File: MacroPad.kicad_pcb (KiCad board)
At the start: 2 copper layers, 111.1 x 120.1 mm, 56 parts, among them J1 AVR-ISP-6, SW1 Rotary_Encoder_Switch, SW10 *, SW11 9, SW12 6, SW13 3, SW14 ., SW15 -, SW16 +, SW17 Enter, SW18 SW_Push, SW2 7, SW3 4, SW4 1, SW5 0, SW6 /, SW7 8, SW8 5, SW9 2, U1 ATmega32U4-AU, U2 PRTR5V0U2X, Y1 16Mhz

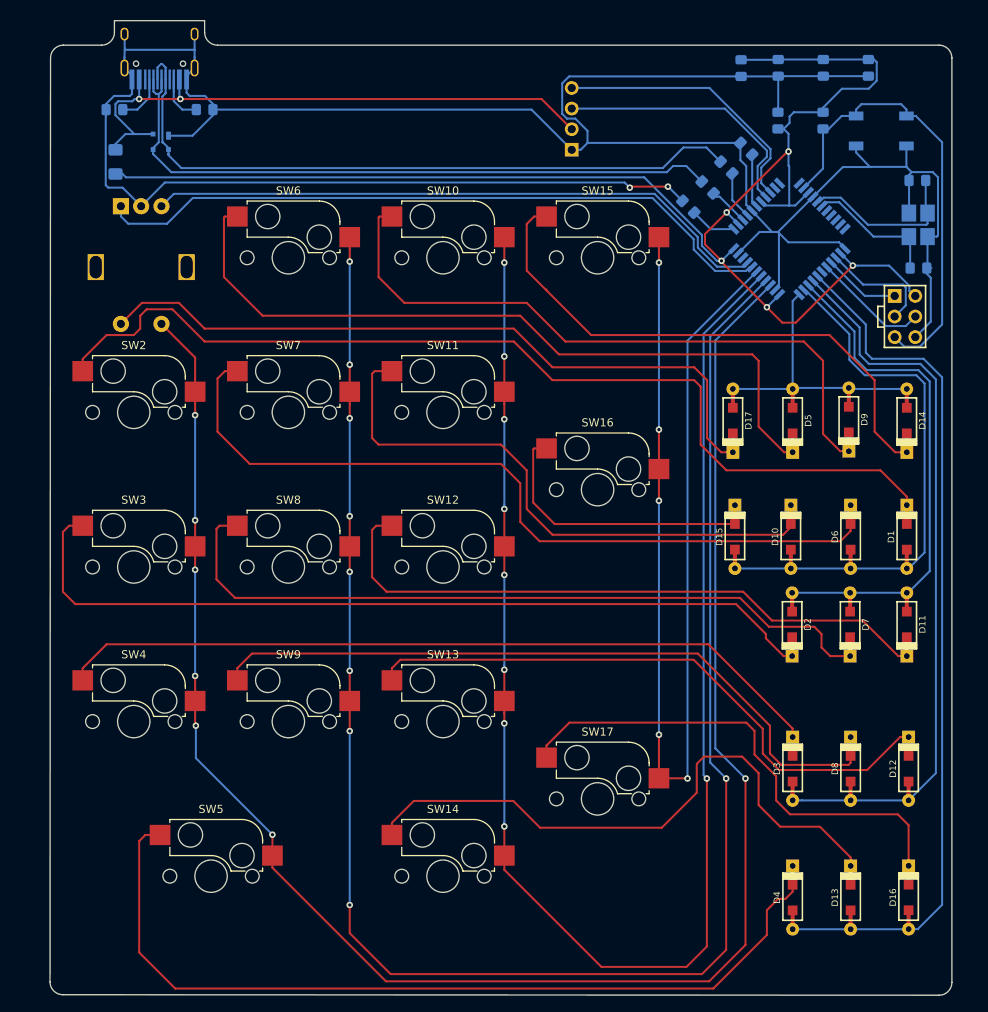
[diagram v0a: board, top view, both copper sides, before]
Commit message: cambiando rutas
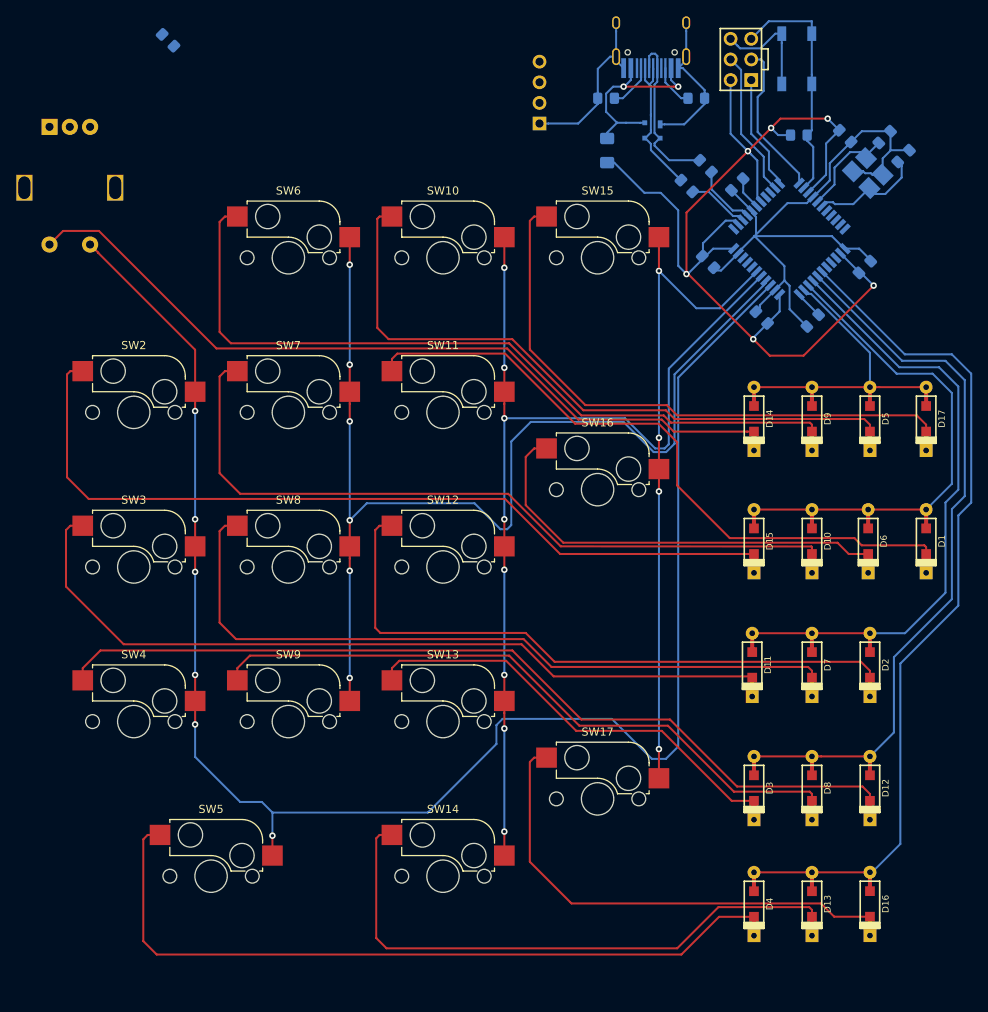
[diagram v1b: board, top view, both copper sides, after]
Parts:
- moved C3 70.7 mm to (54.2, 65.3), turned to 135 degrees
- moved R1 60.6 mm to (119.3, 72.4)
- moved F1 60.6 mm to (108.3, 78.9)
- moved USB1 60.6 mm to (113.8, 60.5)
- moved R2 60.6 mm to (108.2, 72.4)
- moved U2 60.6 mm to (113.9, 76.4)
- moved J1 37.6 mm to (124.8, 67.6), turned to 90 degrees
- moved C2 30.8 mm to (127.4, 99.4), turned to 135 degrees
- moved C5 27.8 mm to (120.8, 92.6), turned to 315 degrees
- moved D17 23.8 mm to (147.6, 111.9)
- moved C4 21.0 mm to (140.1, 93.2), turned to 45 degrees
- moved R6 20.8 mm to (133.7, 99.8), turned to 45 degrees
- moved D11 19.7 mm to (126.2, 142.2)
- moved D14 18.8 mm to (126.4, 111.9)
- moved C6 13.9 mm to (144.9, 79.5), turned to 45 degrees
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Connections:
- net sw14 renamed Net-(D13-Pad1)
- net sw17 renamed Net-(D16-Pad1)
- net sw5 renamed Net-(D4-Pad1)
- net sw8 renamed Net-(D7-Pad1)
- net sw9 renamed Net-(D8-Pad1)
- D1 pad 1: sw2 -> Net-(D1-Pad1)
- D1 pad 2: row1 -> ROW1
- D10 pad 1: sw11 -> Net-(D10-Pad1)
- D10 pad 2: row1 -> ROW1
- D11 pad 1: sw12 -> Net-(D11-Pad1)
- D11 pad 2: row2 -> ROW2
- D12 pad 1: sw13 -> Net-(D12-Pad1)
- D12 pad 2: row3 -> ROW3
- D13 pad 2: row4 -> ROW4
- D14 pad 1: sw15 -> Net-(D14-Pad1)
- D14 pad 2: row0 -> ROW0
- D15 pad 1: sw16 -> Net-(D15-Pad1)
- D15 pad 2: row1 -> ROW1
- D16 pad 2: row4 -> ROW4
- D17 pad 1: S2 -> Net-(D17-Pad1)
- D17 pad 2: row0 -> ROW0
- D2 pad 1: sw3 -> Net-(D2-Pad1)
- D2 pad 2: row2 -> ROW2
- D3 pad 1: sw4 -> Net-(D3-Pad1)
- D3 pad 2: row3 -> ROW3
- D4 pad 2: row4 -> ROW4
- D5 pad 1: sw6 -> Net-(D5-Pad1)
- D5 pad 2: row0 -> ROW0
- D6 pad 1: sw7 -> Net-(D6-Pad1)
- D6 pad 2: row1 -> ROW1
- D7 pad 2: row2 -> ROW2
- D8 pad 2: row3 -> ROW3
- D9 pad 1: sw10 -> Net-(D9-Pad1)
- D9 pad 2: row0 -> ROW0
- SW1 pad S1: col0 -> col3
- SW1 pad S2: S2 -> Net-(D14-Pad1)
- SW10 pad 1: sw10 -> Net-(D5-Pad1)
- SW10 pad 2: col2 -> col1
- SW11 pad 1: sw11 -> Net-(D1-Pad1)
- SW11 pad 2: col2 -> col1
- SW12 pad 1: sw12 -> Net-(D2-Pad1)
- SW12 pad 2: col2 -> col1
- SW13 pad 1: sw13 -> Net-(D3-Pad1)
- SW13 pad 2: col2 -> col1
- SW14 pad 2: col2 -> col1
- SW15 pad 1: sw15 -> Net-(D17-Pad1)
- SW15 pad 2: col3 -> col0
- SW16 pad 1: sw16 -> Net-(D6-Pad1)
- SW16 pad 2: col3 -> col0
- SW17 pad 2: col3 -> col0
- SW2 pad 1: sw2 -> Net-(D15-Pad1)
- SW2 pad 2: col0 -> col3
- SW3 pad 1: sw3 -> Net-(D11-Pad1)
- SW3 pad 2: col0 -> col3
- SW4 pad 1: sw4 -> Net-(D12-Pad1)
- SW4 pad 2: col0 -> col3
- SW5 pad 2: col0 -> col3
- SW6 pad 1: sw6 -> Net-(D9-Pad1)
- SW6 pad 2: col1 -> col2
- SW7 pad 1: sw7 -> Net-(D10-Pad1)
- SW7 pad 2: col1 -> col2
- SW8 pad 2: col1 -> col2
- SW9 pad 2: col1 -> col2
- U1 pad 1: hwb -> Net-(U1-Pad1)
- U1 pad 10: Net-(U1-Pad10) -> mosi
- U1 pad 11: Net-(U1-Pad11) -> sck
- U1 pad 12: Net-(U1-Pad12) -> miso
- U1 pad 25: miso -> Net-(U1-Pad25)
- U1 pad 26: sck -> Net-(U1-Pad26)
- U1 pad 27: mosi -> Net-(U1-Pad27)
- U1 pad 28: Net-(U1-Pad28) -> ROW4
- U1 pad 29: row4 -> ROW3
- U1 pad 30: row3 -> ROW2
- U1 pad 31: row2 -> ROW1
- U1 pad 32: row1 -> ROW0
- U1 pad 33: row0 -> hwb
- U1 pad 36: col0 -> col3
- U1 pad 37: col1 -> col2
- U1 pad 38: col2 -> col1
- U1 pad 39: col3 -> col0
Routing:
- net GND: track 336.6 -> 137.2 mm, vias 2 -> 0
- net col0: track 224.2 -> 82.5 mm, vias 7 -> 4
- net sw2: track 121.3 -> 0.00 mm
- net Net-(D12-Pad1): track 0.00 -> 107.6 mm
- net row4: track 107.2 -> 0.00 mm
- net ROW4: track 0.00 -> 104.6 mm
- net sw3: track 103.6 -> 0.00 mm
- net Net-(D15-Pad1): track 0.00 -> 103.3 mm
- net Net-(D11-Pad1): track 0.00 -> 98.6 mm
- net col1: track 221.6 -> 123.6 mm, vias 9 -> 8
- net Net-(D14-Pad1): track 0.00 -> 97.7 mm
- net sw7: track 97.1 -> 0.00 mm
- net sw4: track 95.5 -> 0.00 mm
- net Net-(D9-Pad1): track 0.00 -> 94.6 mm
- net sw6: track 92.8 -> 0.00 mm
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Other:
- board outline removed
